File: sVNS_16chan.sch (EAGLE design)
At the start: 54 parts, among them IC1 EFM8SB10F8G-A-CSP16R, IC2 OPA990IDCKR, U1 NT3H2211W0FHKH, U2 LT8410EDC-1#TRMPBF, U3 MUX36S16IRSNR, U4 MUX36S16IRSNR

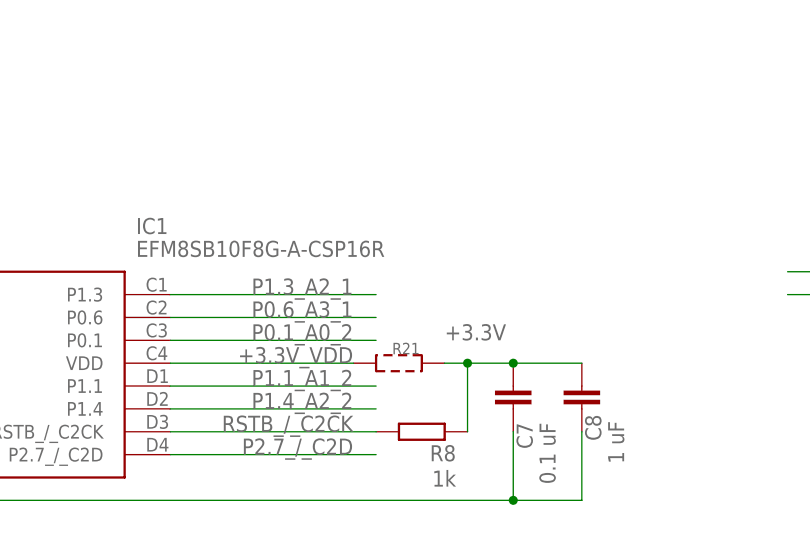
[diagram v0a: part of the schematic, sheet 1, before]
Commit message: Experimentation and routing
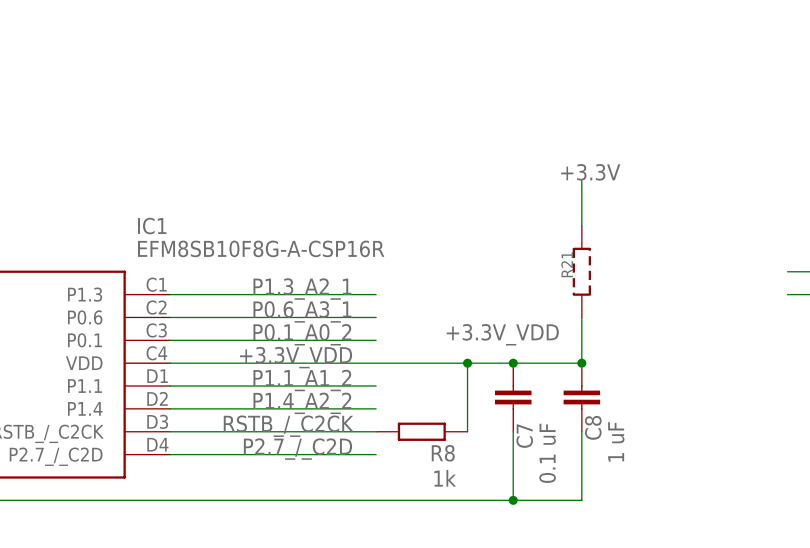
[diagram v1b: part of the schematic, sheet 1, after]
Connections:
- net +3.3V: no longer C7.2, C8.1, R8.1
- net +3.3V_VDD: now also C7.2, C8.1, R8.1
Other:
- moved on the sheet: R21
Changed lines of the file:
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@@
 <part name="R19" library="sVNS_16chan_lib" deviceset="SMD_PADS" device="R0402" package3d_urn="urn:adsk.eagle:package:23547/3"/>
 <part name="R20" library="sVNS_16chan_lib" deviceset="SMD_PADS" device="R0402" package3d_urn="urn:adsk.eagle:package:23547/3"/>
-<part name="R21" library="sVNS_16chan_lib" deviceset="SMD_PADS" device="R0402" package3d_urn="urn:adsk.eagle:package:23547/3"/>
 <part name="R22" library="sVNS_16chan_lib" deviceset="SMD_PADS" device="R0402" package3d_urn="urn:adsk.eagle:package:23547/3"/>
 <part name="R23" library="sVNS_16chan_lib" deviceset="SMD_PADS" device="R0402" package3d_urn="urn:adsk.eagle:package:23547/3"/>
@@
 <part name="JP1" library="sVNS_16chan_lib" deviceset="PINHD-1X1" device="" package3d_urn="urn:adsk.eagle:package:22485/2"/>
 <part name="JP2" library="sVNS_16chan_lib" deviceset="PINHD-1X1" device="" package3d_urn="urn:adsk.eagle:package:22485/2"/>
+<part name="R21" library="sVNS_16chan_lib" deviceset="SMD_PADS" device="R0402" package3d_urn="urn:adsk.eagle:package:23547/3"/>
 </parts>
 <sheets>
@@
 <attribute name="VALUE" x="131.064" y="76.581" size="1.778" layer="96"/>
 </instance>
-<instance part="R21" gate="G$1" x="104.14" y="127" smashed="yes">
-<attribute name="NAME" x="103.378" y="127.9906" size="1.27" layer="95"/>
-<attribute name="VALUE" x="100.33" y="123.698" size="1.778" layer="96"/>
-</instance>
 <instance part="R22" gate="G$1" x="20.32" y="134.62" smashed="yes">
 <attribute name="NAME" x="19.558" y="135.6106" size="1.27" layer="95"/>
@@
 <attribute name="NAME" x="242.57" y="131.445" size="1.778" layer="95" rot="MR180"/>
 <attribute name="VALUE" x="234.95" y="134.62" size="1.778" layer="96" rot="MR180"/>
+</instance>
+<instance part="R21" gate="G$1" x="124.46" y="137.16" smashed="yes" rot="R90">
+<attribute name="NAME" x="123.4694" y="136.398" size="1.27" layer="95" rot="R90"/>
+<attribute name="VALUE" x="127.762" y="133.35" size="1.778" layer="96" rot="R90"/>
 </instance>
 </instances>
@@
 </segment>
 <segment>
-<pinref part="C8" gate="G$1" pin="1"/>
-<wire x1="124.46" y1="127" x2="116.84" y2="127" width="0.1524" layer="91"/>
-<pinref part="C7" gate="G$1" pin="2"/>
-<junction x="116.84" y="127"/>
-<wire x1="116.84" y1="127" x2="111.76" y2="127" width="0.1524" layer="91"/>
-<pinref part="R8" gate="G$1" pin="1"/>
-<wire x1="111.76" y1="119.38" x2="111.76" y2="127" width="0.1524" layer="91"/>
-<junction x="111.76" y="127"/>
-<wire x1="111.76" y1="127" x2="109.22" y2="127" width="0.1524" layer="91"/>
-<label x="109.22" y="129.54" size="1.778" layer="95"/>
-<pinref part="R21" gate="G$1" pin="2"/>
-</segment>
-<segment>
 <junction x="58.42" y="73.66"/>
 <wire x1="58.42" y1="73.66" x2="58.42" y2="88.9" width="0.1524" layer="91"/>
@@
 <wire x1="58.42" y1="73.66" x2="55.88" y2="73.66" width="0.1524" layer="91"/>
 <pinref part="R23" gate="G$1" pin="2"/>
+</segment>
+<segment>
+<pinref part="R21" gate="G$1" pin="2"/>
+<wire x1="124.46" y1="142.24" x2="124.46" y2="147.32" width="0.1524" layer="91"/>
+<label x="121.92" y="147.32" size="1.778" layer="95"/>
 </segment>
 </net>
@@
 <net name="+3.3V_VDD" class="0">
 <segment>
+<pinref part="C7" gate="G$1" pin="2"/>
+<wire x1="116.84" y1="127" x2="111.76" y2="127" width="0.1524" layer="91"/>
+<pinref part="R8" gate="G$1" pin="1"/>
+<wire x1="111.76" y1="119.38" x2="111.76" y2="127" width="0.1524" layer="91"/>
+<junction x="111.76" y="127"/>
+<label x="109.22" y="129.54" size="1.778" layer="95"/>
 <pinref part="IC1" gate="G$1" pin="VDD"/>
 <label x="99.06" y="127" size="1.778" layer="95" align="bottom-right"/>
-<wire x1="99.06" y1="127" x2="78.74" y2="127" width="0.1524" layer="91"/>
+<wire x1="111.76" y1="127" x2="78.74" y2="127" width="0.1524" layer="91"/>
+<pinref part="C8" gate="G$1" pin="1"/>
 <pinref part="R21" gate="G$1" pin="1"/>
-</segment>
-</net>
+<wire x1="124.46" y1="132.08" x2="124.46" y2="127" width="0.1524" layer="91"/>
+<wire x1="124.46" y1="127" x2="116.84" y2="127" width="0.1524" layer="91"/>
+<junction x="124.46" y="127"/>
+<junction x="116.84" y="127"/>
+</segment>
+</net>
